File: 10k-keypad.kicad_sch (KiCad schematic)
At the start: 62 parts, among them J1 AVR-ISP-6, K1 SW_Push, K10 SW_Push, K2 SW_Push, K3 SW_Push, K4 SW_Push, K5 SW_Push, K6 SW_Push, K7 SW_Push, K8 SW_Push, K9 SW_Push, SW1 SW_Push, U1 ATmega32U4-M, U2 DRV5055A2xDBZxQ1, U3 DRV5055A2xDBZxQ1, U4 DRV5055A2xDBZxQ1, U5 DRV5055A2xDBZxQ1, U6 DRV5055A2xDBZxQ1, Y1 Crystal_GND24_Small

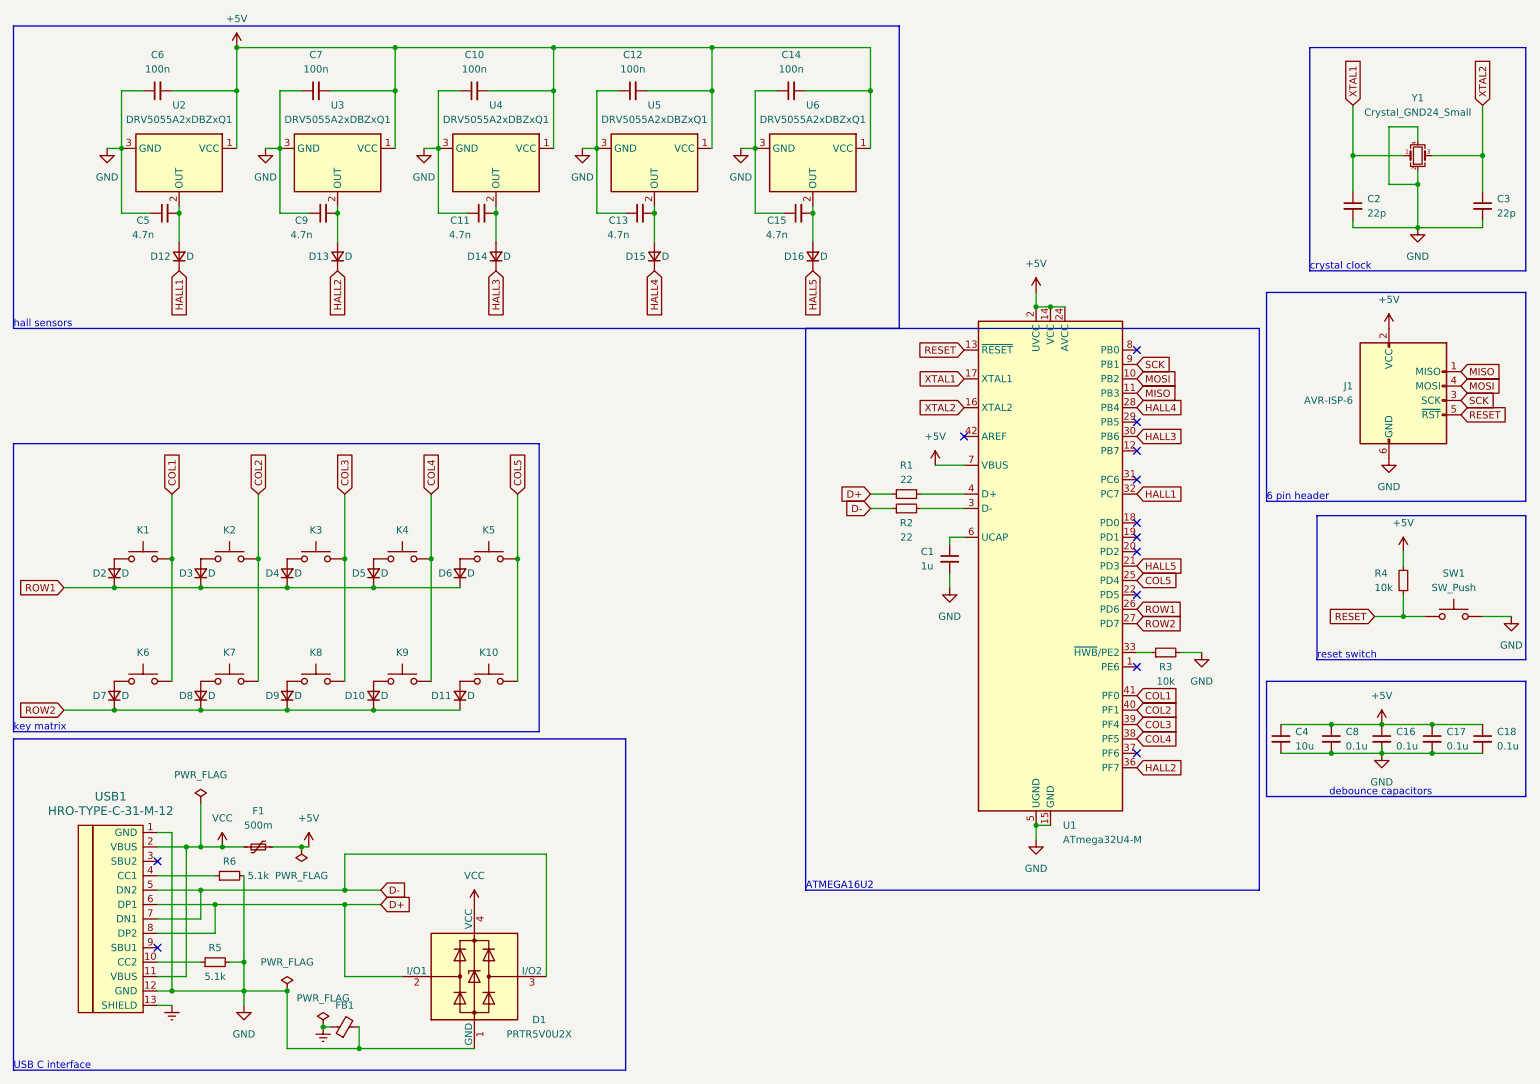
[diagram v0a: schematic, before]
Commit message: fix schematic, gerbers
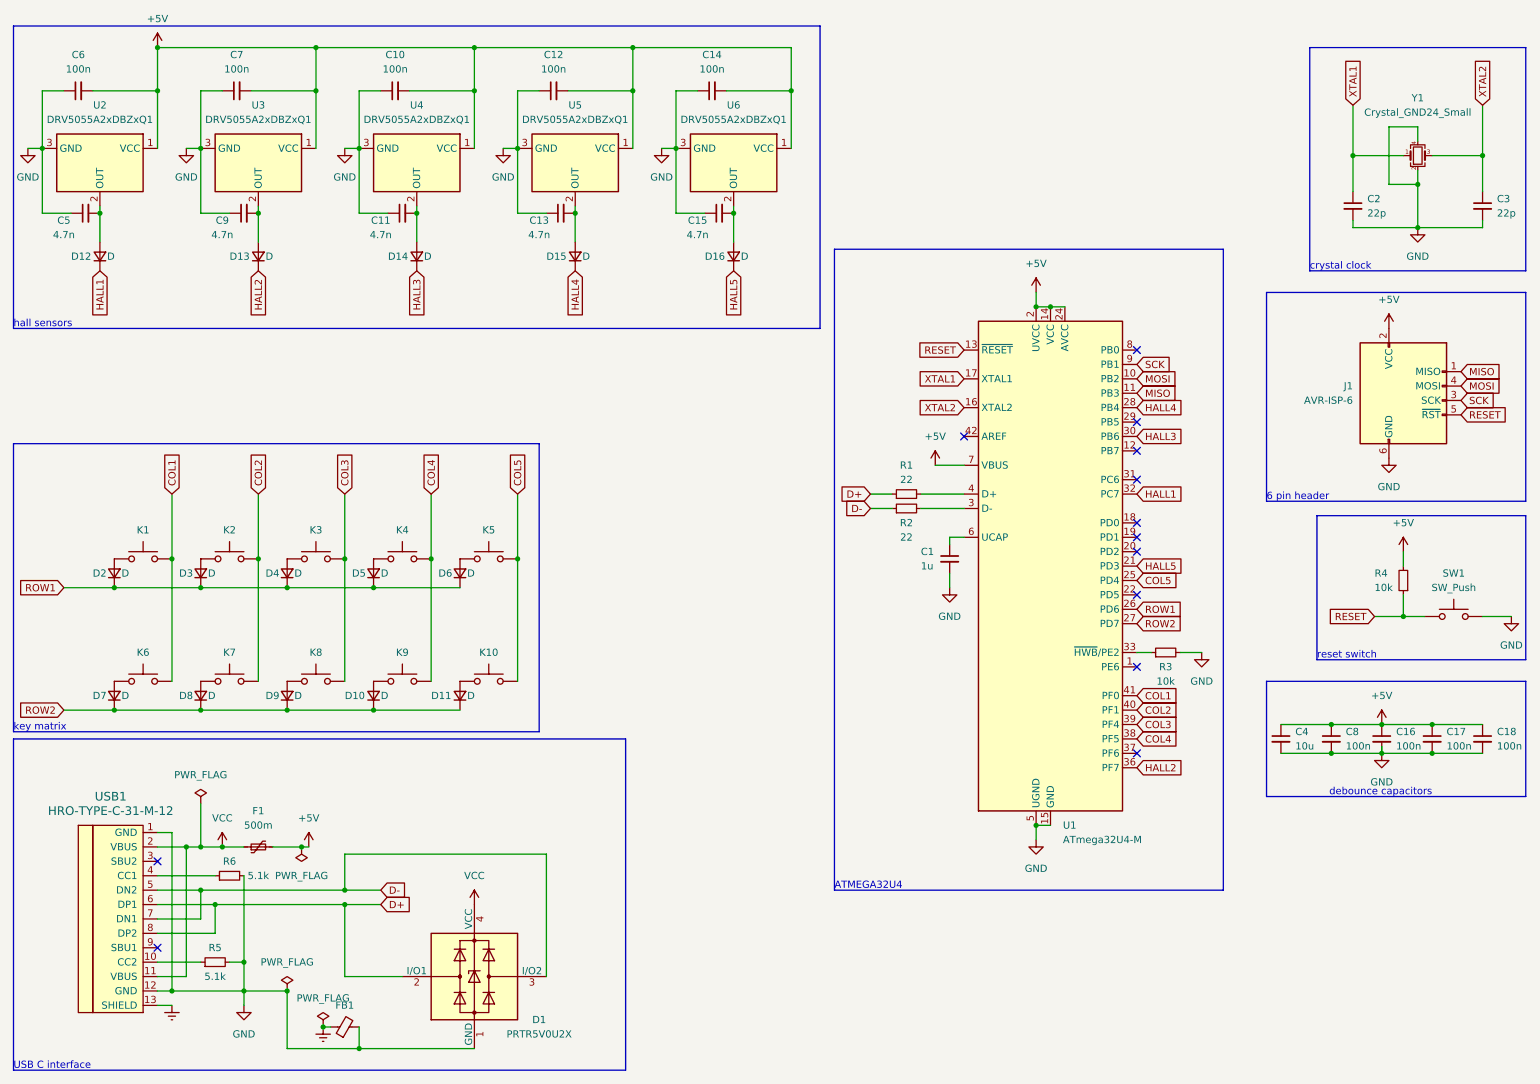
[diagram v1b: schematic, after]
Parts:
- C16, C17, C18, C8: value 0.1u -> 100n
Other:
- note added: "ATMEGA32U4"
- note removed: "ATMEGA16U2"
- moved on the sheet: C10, C11, C12, C13, C14, C15, C5, C6, C7, C9, D12, D13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
